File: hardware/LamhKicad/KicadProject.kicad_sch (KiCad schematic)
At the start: 28 parts, among them J2 ESQ-110-X-X-D, J3 2060-1452/998-404, J4 Conn_02x03_Odd_Even, U1 TJA1051T-3, U2 PCA9745BTW, U3 TLV70433DBVT, U4 INA180A3, U5 STM32F072C8Tx

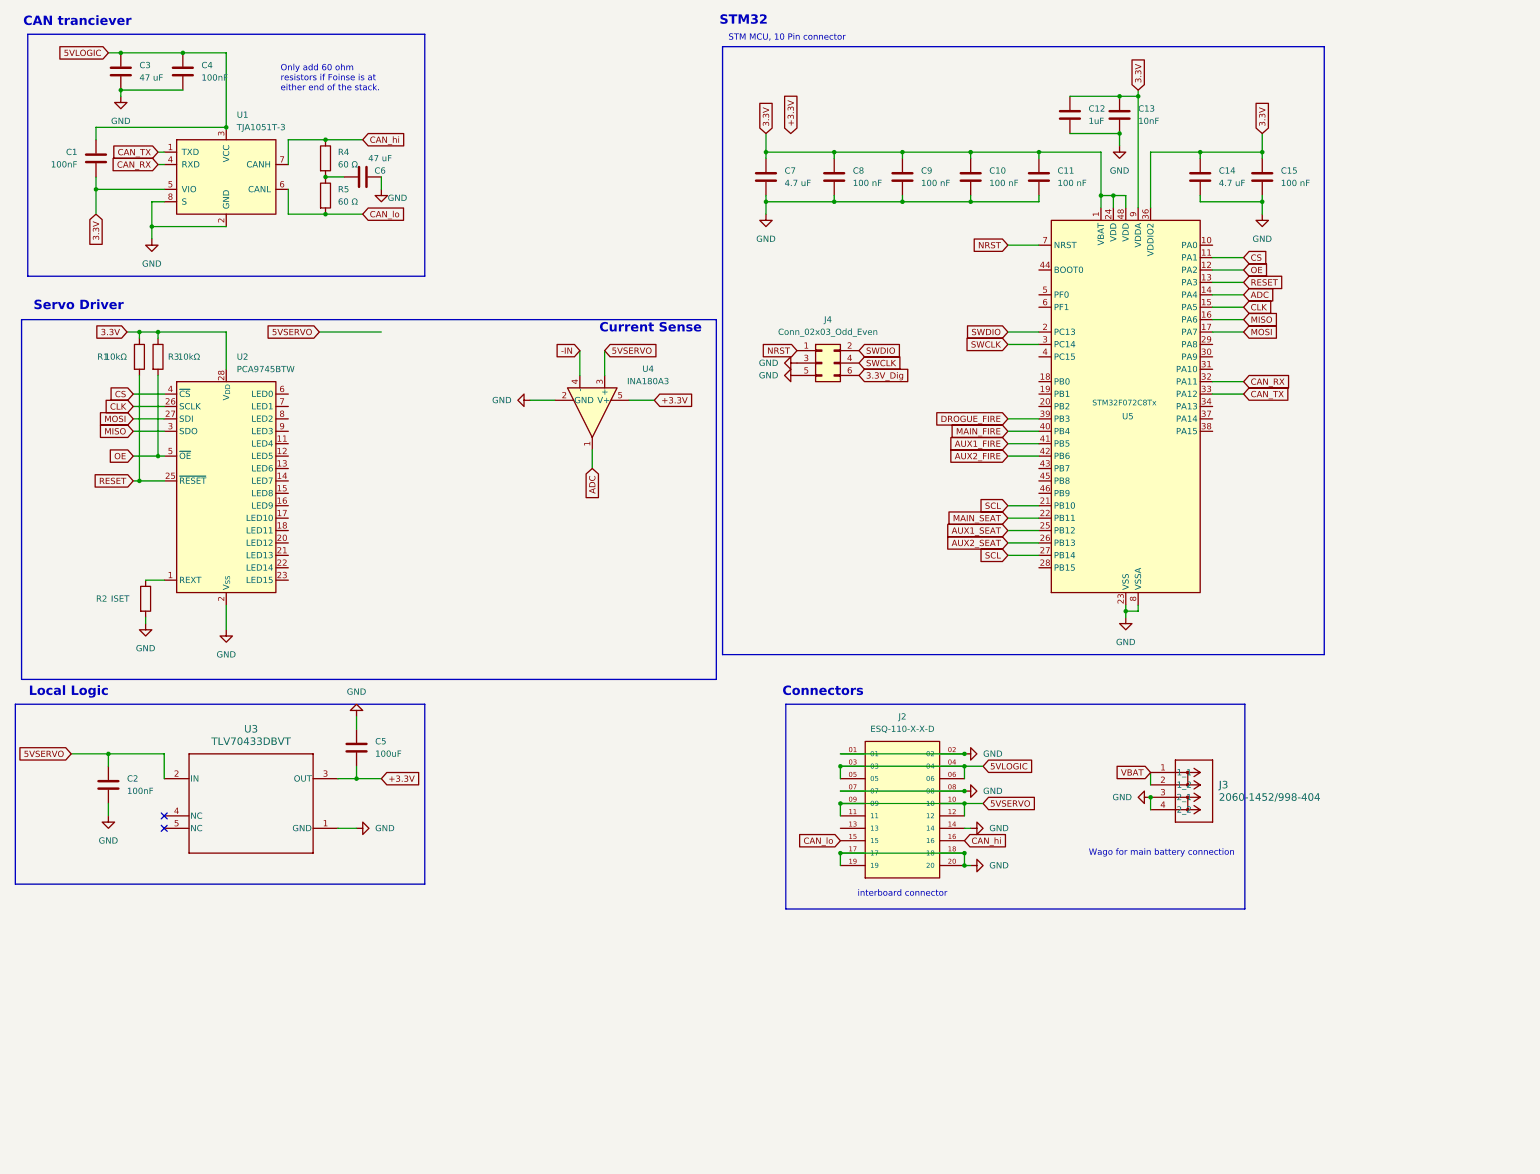
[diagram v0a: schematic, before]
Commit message: started
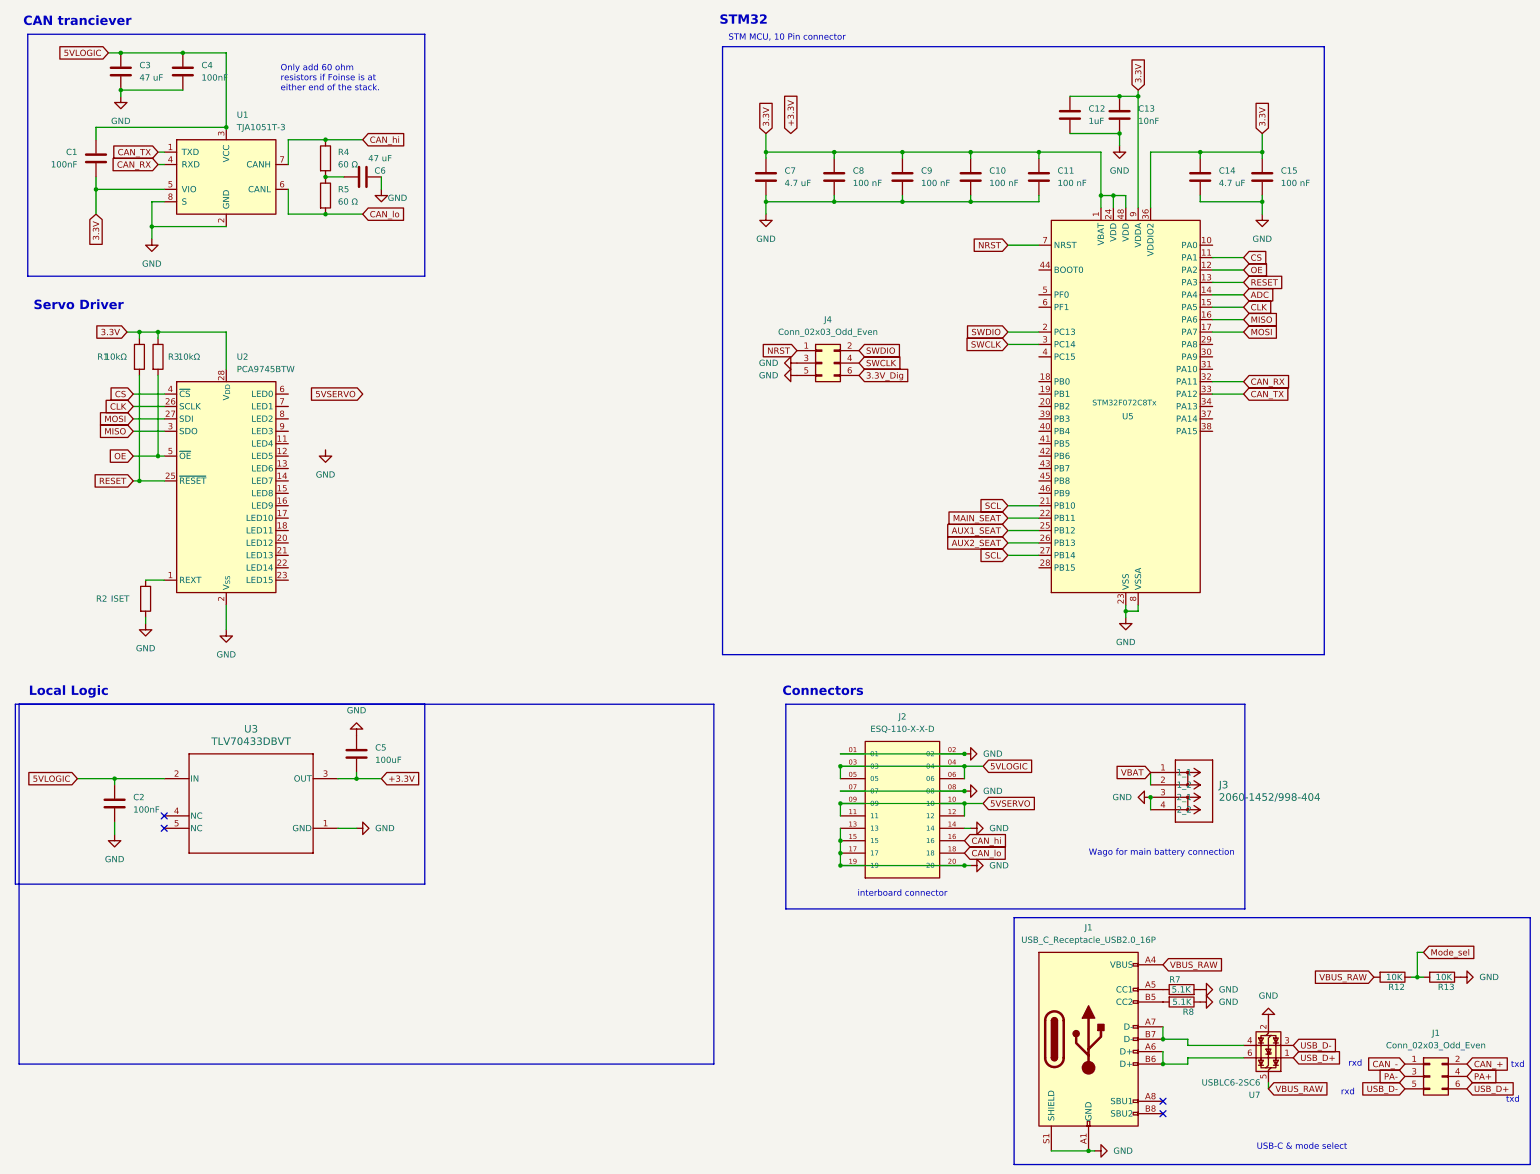
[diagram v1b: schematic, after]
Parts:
- removed U4: INA180A3, Package_TO_SOT_SMD:SOT-23-5, symbol Amplifier_Current:INA180A3
- added J1: USB_C_Receptacle_USB2.0_16P, Connector_USB:USB_C_Receptacle_G-Switch_GT-USB-7010ASV, symbol Connector:USB_C_Receptacle_USB2.0_16P
- added J1: Conn_02x03_Odd_Even, Connector_PinHeader_1.00mm:PinHeader_2x03_P1.00mm_Vertical, symbol Connector_Generic:Conn_02x03_Odd_Even
- added R12, R13: 10K, Resistor_SMD:R_0402_1005Metric, symbol Device:R
- added R7, R8: 5.1K, Resistor_SMD:R_0402_1005Metric, symbol Device:R
- added U7: USBLC6-2SC6, Package_TO_SOT_SMD:SOT-23-6, symbol Power_Protection:USBLC6-2SC6
- R1, R2, R3, R4, R5: footprint Capacitor_SMD:C_0402_1005Metric -> Resistor_SMD:R_0402_1005Metric
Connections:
- net 5VLOGIC: now also C2.1, U3.2 (IN)
- net 5VSERVO: no longer C2.1, U3.2 (IN)
- net CAN_lo: now also J2.18; no longer J2.15
- net GND: now also J2.13, J2.15, J1.A1 (GND), J1.A12 (GND), J1.B1 (GND), J1.B12 (GND), J1.S1 (SHIELD), R13.1, R7.2, R8.1, U7.2 (GND); no longer J2.18
- net AUX1_FIRE: no longer names the net of U5.41 (PB5)
- net AUX2_FIRE: no longer names the net of U5.42 (PB6)
- net DROGUE_FIRE: no longer names the net of U5.39 (PB3)
- net MAIN_FIRE: no longer names the net of U5.40 (PB4)
- new net: J1.A7 (D-), J1.B7 (D-), U7.4 (I/O2)
- new net: J1.A6 (D+), J1.B6 (D+), U7.6 (I/O1)
- new net: J1.B5 (CC2), R8.2
- new net: J1.A5 (CC1), R7.1
- new net CAN_+: J1.2 (Pin_2)
- new net CAN_-: J1.1 (Pin_1)
- new net Mode_sel: R12.1, R13.2
- new net PA+: J1.4 (Pin_4)
- new net PA-: J1.3 (Pin_3)
- new net USB_D+: J1.6 (Pin_6), U7.1 (I/O1)
- new net USB_D-: J1.5 (Pin_5), U7.3 (I/O2)
- new net VBUS_RAW: J1.A4 (VBUS), J1.A9 (VBUS), J1.B4 (VBUS), J1.B9 (VBUS), R12.2, U7.5 (VBUS)
- no-connect marks 2 -> 4
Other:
- note added: "USB-C & mode select"
- note added: "rxd"
- note added: "txd"
- note removed: "Current Sense"
- moved on the sheet: C2, C5
